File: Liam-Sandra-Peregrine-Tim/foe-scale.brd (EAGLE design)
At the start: 100 x 80 mm, 40 parts, among them U1 LM311, U2 SAMD21E, U3 3.3V_AS1363

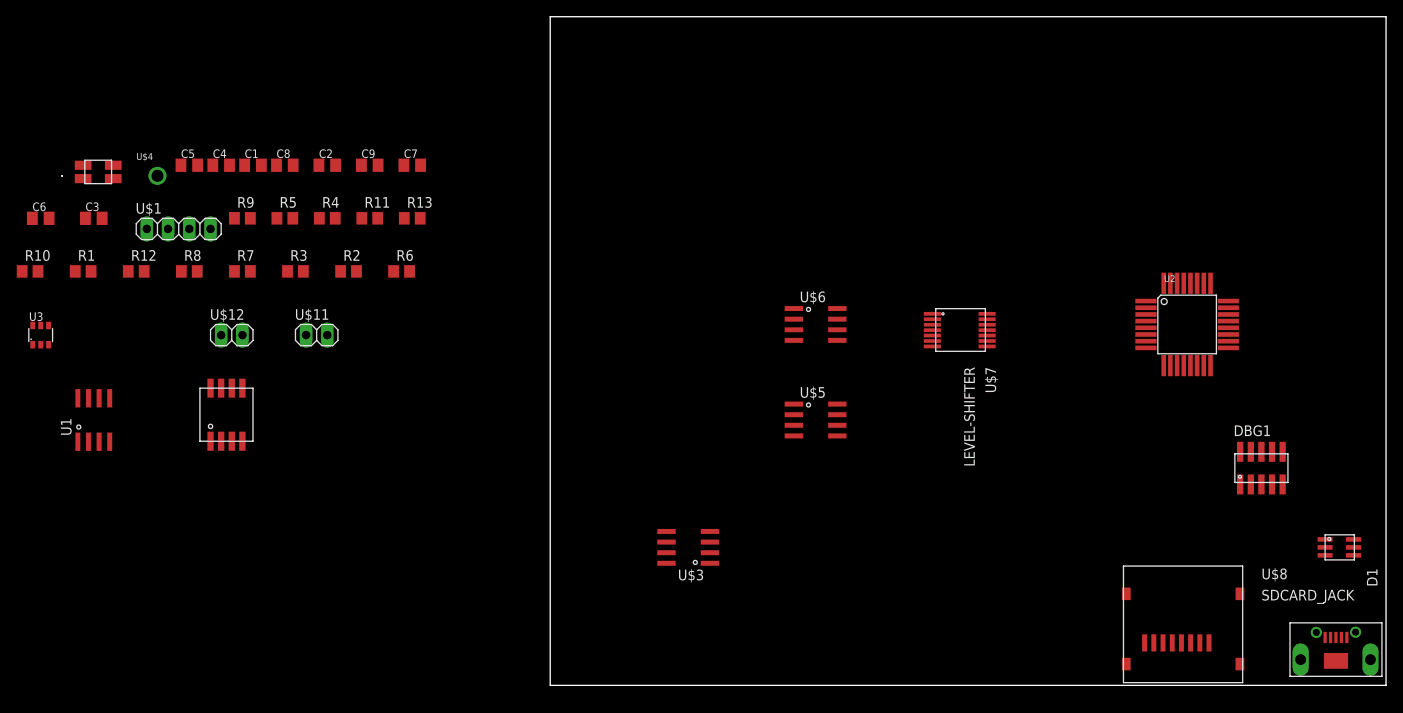
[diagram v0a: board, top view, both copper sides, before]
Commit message: finished up schematic
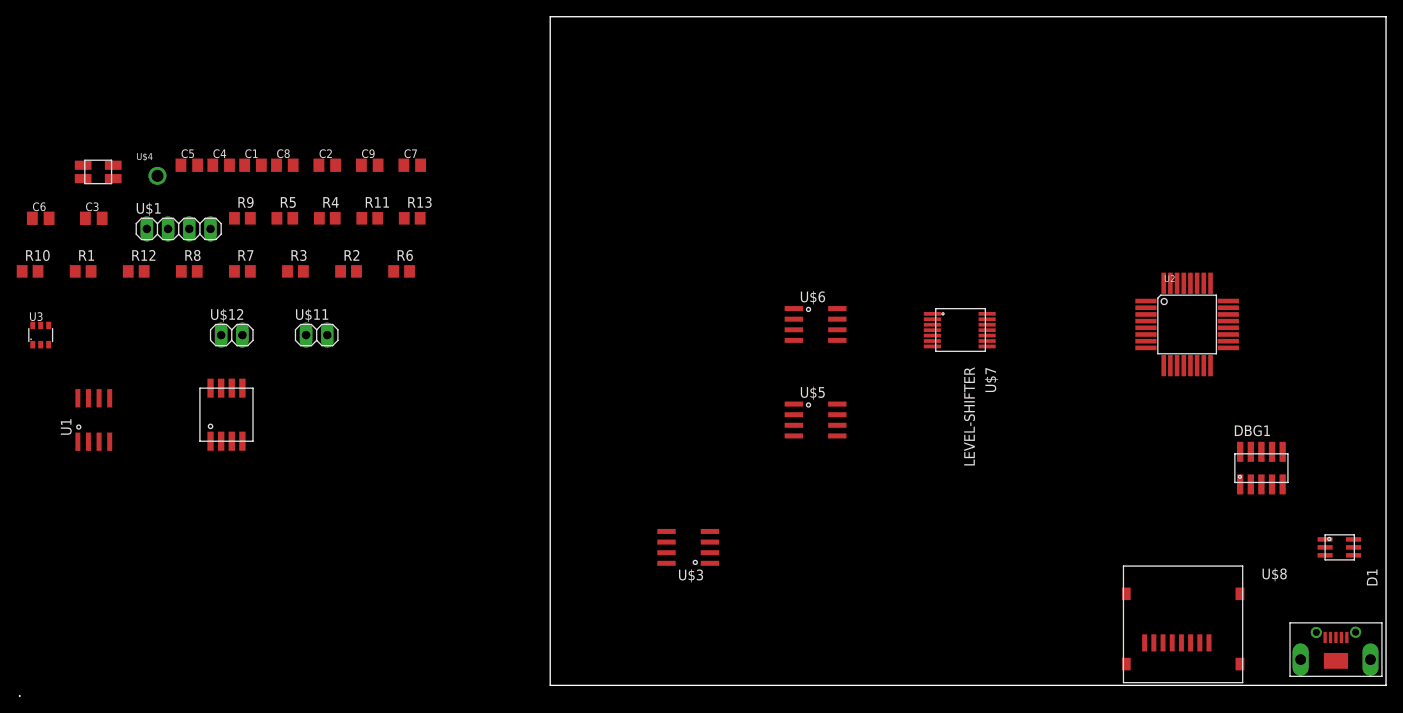
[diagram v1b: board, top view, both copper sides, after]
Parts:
- U$8: value SDCARD_JACK -> (none); device test:MICRO_SDCARD -> foe-scale:MICRO_SDCARD
- U$9: device test:RED_LED -> foe-scale:RED_LED
- moved U$9 62.4 mm to (-63.5, -1.27)
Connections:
- net N$40 renamed +3.3V
- removed net /SAMPLE-PA01: U1.7
- removed net N$1: U$1.1
- removed net N$11: R3.1
- removed net N$12: R2.2
- removed net N$13: U$3.8
- removed net N$14: U$3.4
- removed net N$15: U$2.+VS
- removed net N$17: C2.2
- removed net N$21: C1.2
- removed net N$22: R7.1
- removed net N$24: R8.2
- removed net N$25: C4.2
- removed net N$26: U1.1
- removed net N$28: C5.2
- removed net N$29: U1.4
- removed net N$30: U1.8
- removed net N$31: U2.26
- removed net N$32: C6.2
- removed net N$33: U$6.3, U$6.4
- removed net N$37: U$6.8
- removed net N$38: U$7.VL
- removed net N$39: U$7.GND, U$7.IVL4
- removed net N$4: U$1.4
- removed net N$41: U$13.GND
- removed net N$42: D1.CH2, U$13.D-
- removed net N$43: D1.CH1, U$13.D+
- removed net N$44: U2.28
- removed net N$47: U$10.A
- removed net N$51: U2.17
- removed net N$52: U2.18
- removed net N$53: U2.19
- removed net N$54: U2.20
- removed net N$55: U2.11
- removed net N$56: U2.12
- removed net N$57: U2.13
- removed net N$58: U2.14
- removed net N$59: U2.30
- removed net N$60: U2.10
- removed net N$61: U2.3
- removed net N$62: U2.9
- removed net N$63: C8.1, R11.1, U3.1
- removed net N$66: C8.2
- removed net N$68: C9.2, U3.6
- removed net N$69: DBG1.VREF
- removed net N$71: U3.4
- removed net N$72: R13.2
- removed net N$73: R13.1
- removed net N$74: DBG1.DGND1, DBG1.DGND2
- removed net N$75: DBG1.SWDIO
- removed net N$76: DBG1.SWDCLK
- removed net N$77: D1.V_N
- removed net N$78: D1.V_P
- removed net N$79: DBG1.NRESET
- removed net N$8: U$2.–VS
- new net /SAMPLE-PA11: U1.7, U2.14
- net +5V: now also C8.1, D1.V_P, R11.1, R2.2, R7.1, U$1.1, U$2.+VS, U$3.8, U$6.8, U$7.VL, U1.8, U3.1; no longer U$9.P+
- net 3.3V: now also C9.2, DBG1.VREF, U$10.A, U$8.VDD, U2.30, U2.9, U3.6; no longer U$8.P4
- net AGND: now also C1.2, C2.2, C4.2, C5.2, R13.2, R3.1, R8.2, U$1.4, U$2.–VS, U$3.4, U$6.3, U$6.4, U$7.GND, U$7.IVL4, U1.1, U1.4; no longer U$9.P-
- net CLK-PA17: now also U$8.CLK, U2.18; no longer U$8.P5
- net CONV-PA10: now also U2.13
- net CS-PA19: now also U$8.CD, U2.20; no longer U$8.P2
- net DGND: now also C6.2, C8.2, D1.V_N, DBG1.DGND1, DBG1.DGND2, R13.1, U$13.GND, U$8.VSS, U2.10, U2.28, U3.4; no longer U$8.P6
- net DI-PA18: now also U$8.CMD, U2.19; no longer U$8.P3
- net DO-PA16: now also U$8.DAT0, U2.17; no longer U$8.P7
- net HYS-PA02: now also U2.3
- net RST: now also DBG1.NRESET, U2.26
- net SCK-PA08: now also U2.11
- net SDO-PA09: now also U2.12
- net SWDCLK: now also DBG1.SWDCLK
- net SWDIO: now also DBG1.SWDIO
- net USB_D+_PA25: now also D1.CH1, U$13.D+
- net USB_D-_PA24: now also D1.CH2, U$13.D-
